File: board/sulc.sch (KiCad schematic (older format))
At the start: 64 parts, among them J1 LED_PWR, J2 HWB, P1 USB, P10 CONN_1, P11 CONN_1, P12 CONN_1, P13 CONN_1, P14 CONN_1, P15 CONN_1, P16 CONN_1, P17 CONN_1, P18 CONN_1, P19 CONN_1, P2 CONN_1, P20 CONN_1, P21 CONN_1, P22 CONN_1, P23 CONN_1, P24 CONN_1, P25 CONN_1, P3 CONN_1, P4 CONN_1, P5 CONN_1, P6 CONN_1, P7 ISP, P8 CONN_1, P9 CONN_1, U1 ATMEGA8U2AU, Y1 16MHz

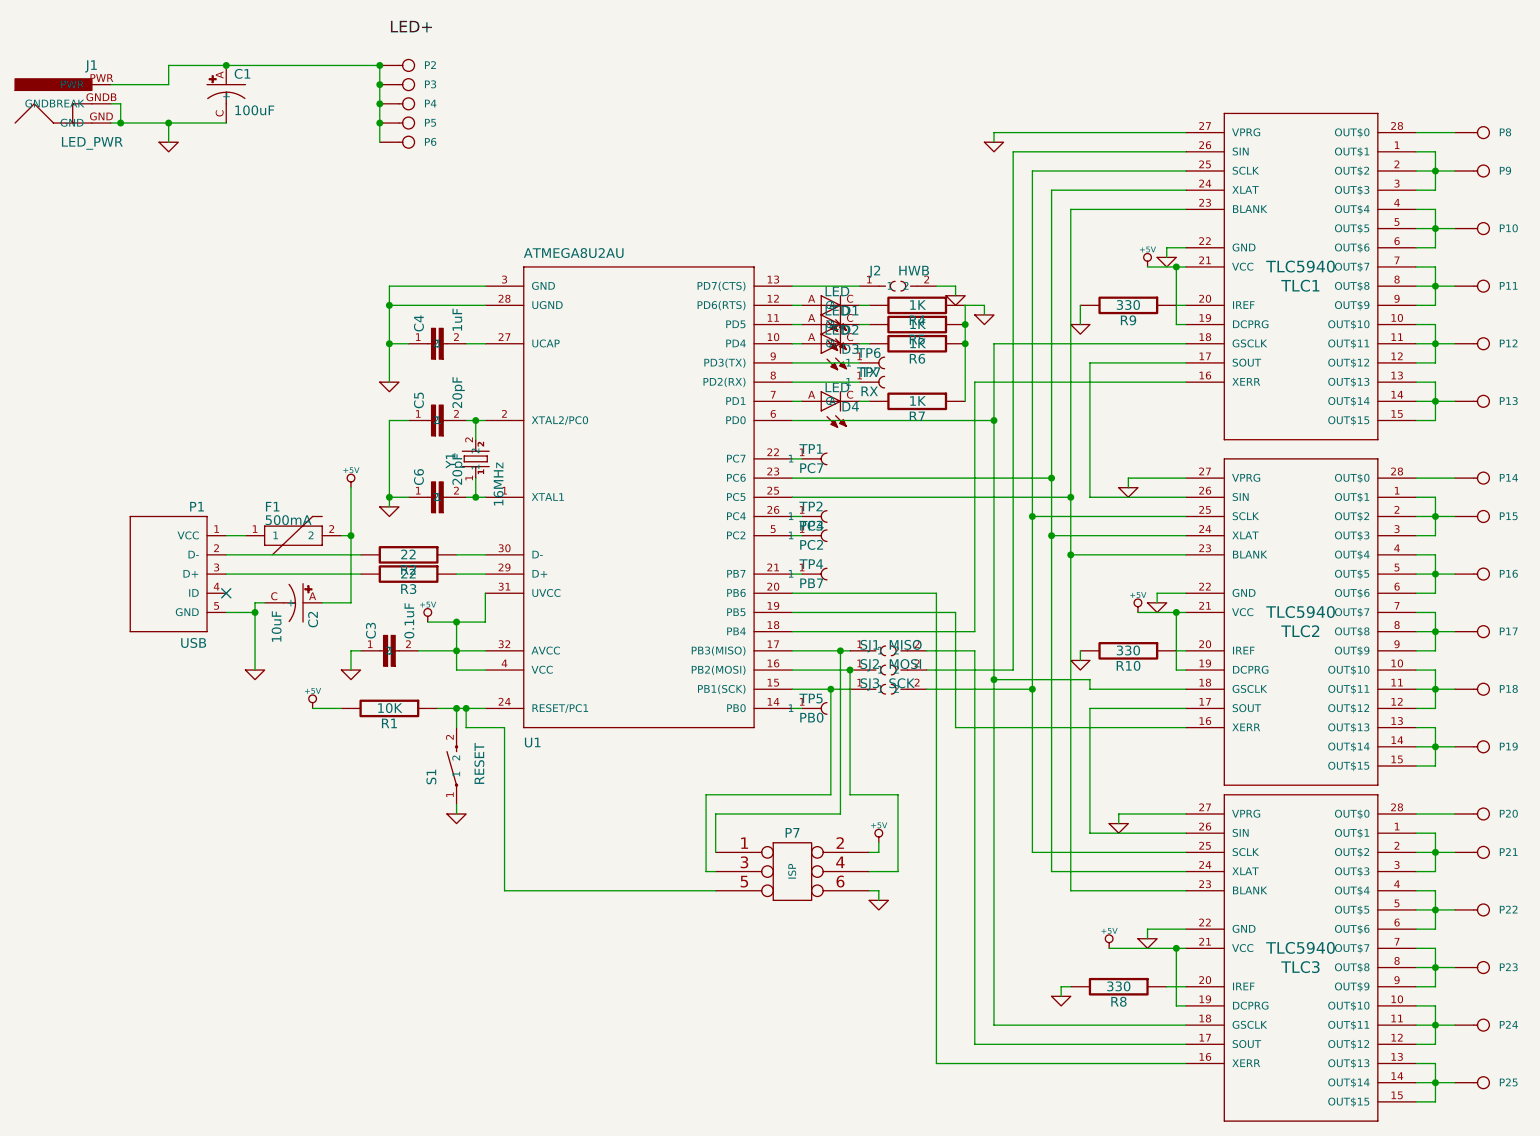
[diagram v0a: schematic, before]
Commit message: Preliminary PCB design
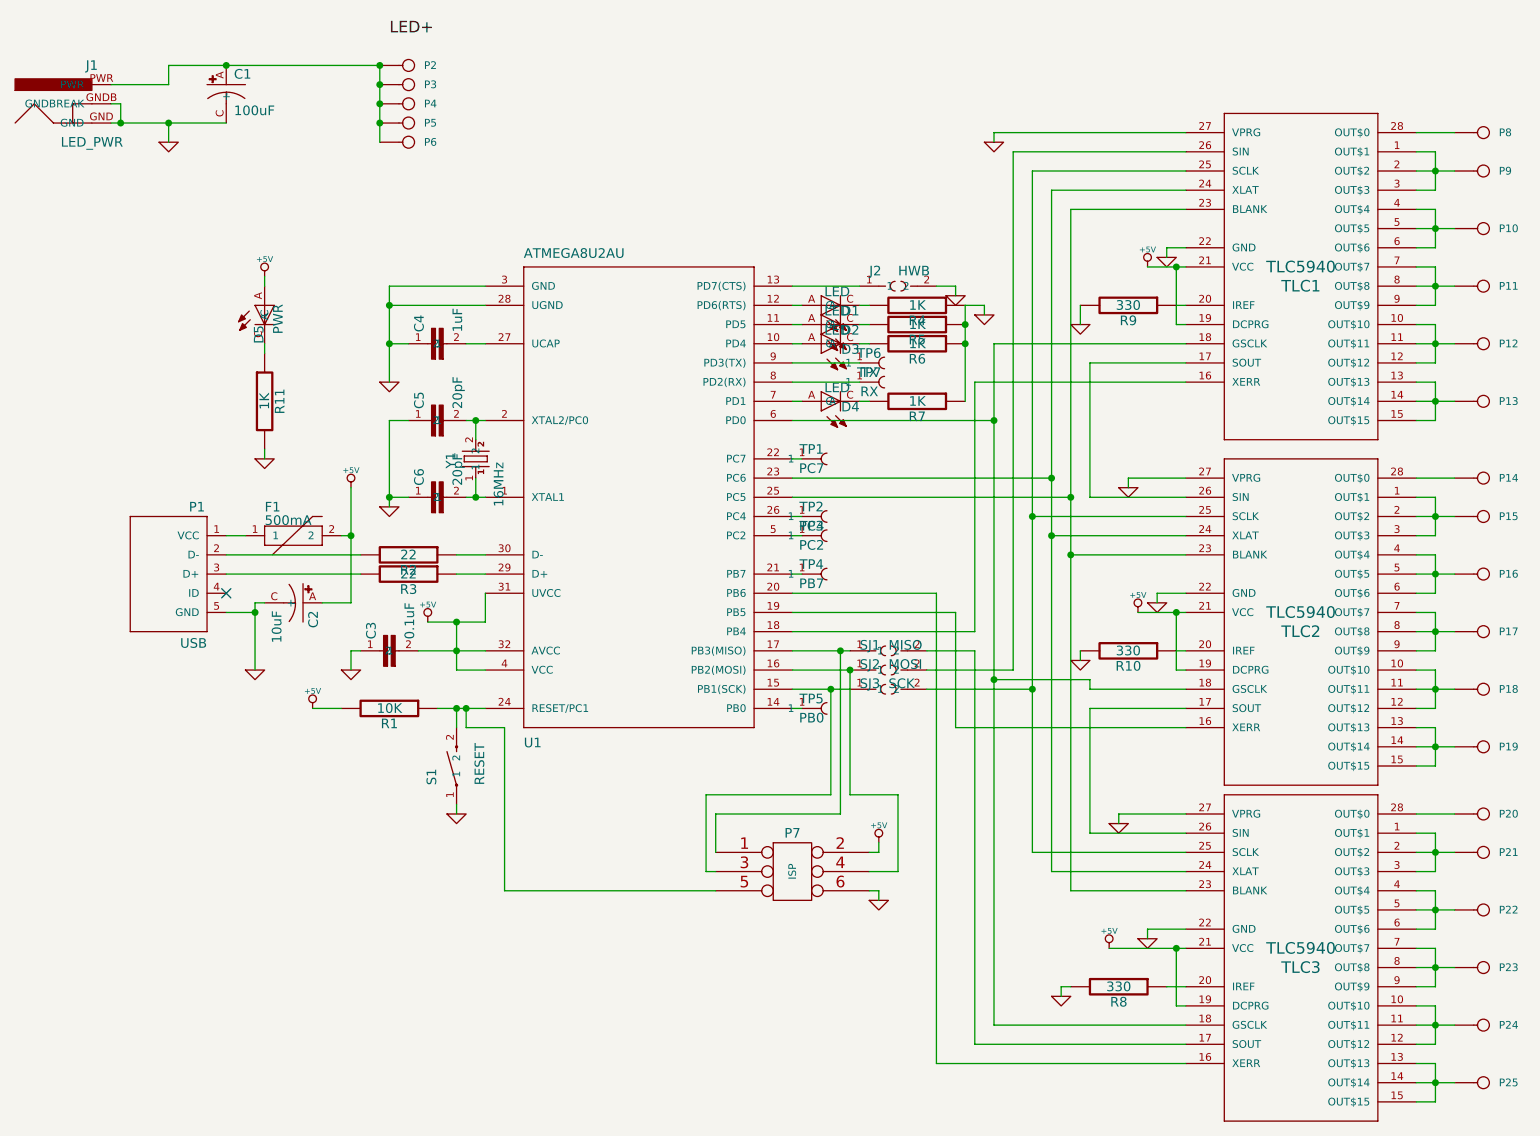
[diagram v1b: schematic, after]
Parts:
- added D5: PWR, SparkFun-LED-1206, symbol LED1206
- added R11: 1K, symbol R
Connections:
- net +5V: now also D5.A
- net GND: now also R11.2
- new net: D5.C, R11.1
